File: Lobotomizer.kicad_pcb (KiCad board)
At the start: 2 copper layers, 134 x 101.6 mm, 170 parts, among them J1 IN, J2 OUT, J3 Barrel_Jack, Q1 NTE467, Q2 2N5089, Q201 MPSA05, Q202 MPSA05, Q3 2N5087, Q4 2N5089, Q5 NTE467, Q6 BS170, SW1 SW_SPDT_MSM, SW101 SW_Push_DPDT, SW102 SW_SPDT, SW2 SW_SPDT, SW201 SW_SPDT, SW202 SW_SPDT, SW3 SW_SPDT, U1 LM741, U101 TLC27M4AIN, U102 BTDR-2H-L, U103 L7805, U201 LM386, U202 TL072

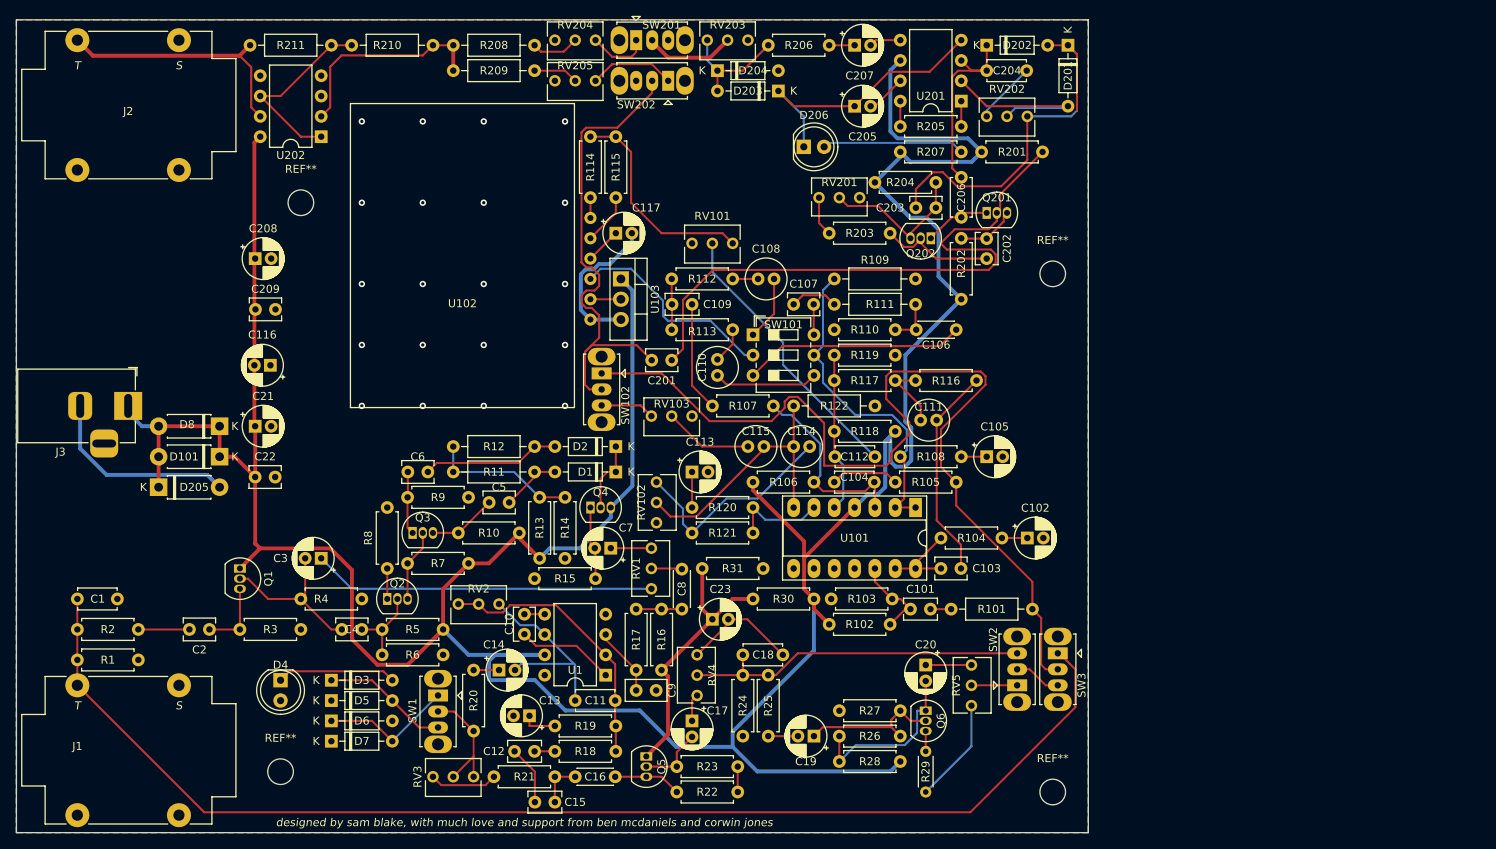
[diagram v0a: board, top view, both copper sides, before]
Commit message: lobotomizer v2 update
so much changed i cant note it all here
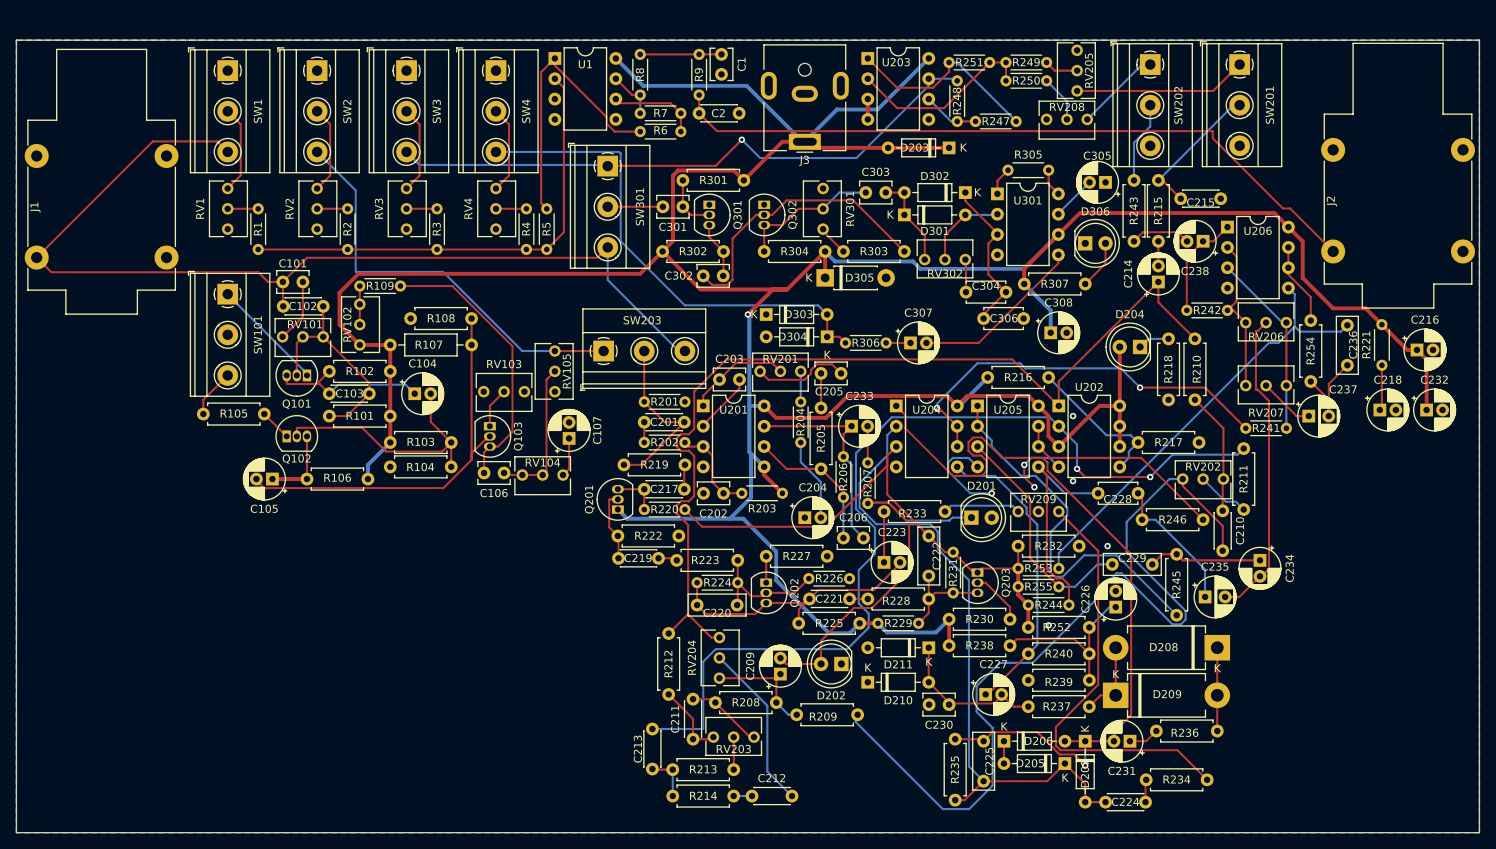
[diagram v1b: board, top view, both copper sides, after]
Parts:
- removed C10: 30p, Capacitor_THT:C_Rect_L4.0mm_W2.5mm_P2.50mm
- removed C108, C110, C115: 220n, Capacitor_THT:C_Radial_D5.0mm_H11.0mm_P2.00mm
- removed C109: 33n, Capacitor_THT:C_Rect_L4.0mm_W2.5mm_P2.50mm
- removed C11, C18: 100p, Capacitor_THT:C_Disc_D4.7mm_W2.5mm_P5.00mm
- removed C111, C114: 470p, Capacitor_THT:C_Radial_D5.0mm_H11.0mm_P2.00mm
- removed C112: 10n, Capacitor_THT:C_Disc_D4.7mm_W2.5mm_P5.00mm
- removed C113, C17, C19, C3, C7: 1u, Capacitor_THT:CP_Radial_D5.0mm_P2.00mm
- removed C116, C117, C207, C208, C21: 100u, Capacitor_THT:CP_Radial_D5.0mm_P2.00mm
- removed C12: 2.2p, Capacitor_THT:C_Rect_L4.0mm_W2.5mm_P2.50mm
- removed C13, C14: 4.7u, Capacitor_THT:CP_Radial_D5.0mm_P2.00mm
- removed C15: 3.3n, Capacitor_THT:C_Rect_L4.0mm_W2.5mm_P2.50mm
- removed C16, C8: 22n, Capacitor_THT:C_Disc_D4.3mm_W1.9mm_P5.00mm
- removed C20, C23: 10u, Capacitor_THT:CP_Radial_D5.0mm_P2.00mm
- removed C22, C4, C5, C6: 100n, Capacitor_THT:C_Disc_D3.8mm_W2.6mm_P2.50mm
- removed C9: 1n, Capacitor_THT:C_Disc_D5.0mm_W2.5mm_P2.50mm
- removed D1, D2, D3, D5, D6, D7: 4148, Diode_THT:D_DO-35_SOD27_P7.62mm_Horizontal
- removed D101: 4001, Diode_THT:D_DO-41_SOD81_P7.62mm_Horizontal
- removed D4: LED, LED_THT:LED_D5.0mm
- removed D8: 5817, Diode_THT:D_DO-41_SOD81_P7.62mm_Horizontal
- removed G***: LOGO, BSilk:Lobotomizer
- removed Q1, Q5: NTE467, Package_TO_SOT_THT:TO-92_Inline
- removed Q2, Q4: 2N5089, Package_TO_SOT_THT:TO-92_Inline
- removed Q3: 2N5087, Package_TO_SOT_THT:TO-92_Inline
- removed Q6: BS170, Package_TO_SOT_THT:TO-92_Inline
- removed R10, R120, R15, R23, R28, R30, R31: 10K, Resistor_THT:R_Axial_DIN0207_L6.3mm_D2.5mm_P7.62mm_Horizontal
- removed R11, R111, R12, R122: 100K, Resistor_THT:R_Axial_DIN0207_L6.3mm_D2.5mm_P10.16mm_Horizontal
- removed R110, R17, R20, R25: 1K, Resistor_THT:R_Axial_DIN0207_L6.3mm_D2.5mm_P7.62mm_Horizontal
- removed R112, R113: 39K, Resistor_THT:R_Axial_DIN0207_L6.3mm_D2.5mm_P7.62mm_Horizontal
- removed R114, R115: 5K, Resistor_THT:R_Axial_DIN0207_L6.3mm_D2.5mm_P7.62mm_Horizontal
- removed R116, R118, R119, R16, R22, R24: 1M, Resistor_THT:R_Axial_DIN0207_L6.3mm_D2.5mm_P7.62mm_Horizontal
- removed R117: 6.8K, Resistor_THT:R_Axial_DIN0207_L6.3mm_D2.5mm_P7.62mm_Horizontal
- removed R121: 68K, Resistor_THT:R_Axial_DIN0207_L6.3mm_D2.5mm_P7.62mm_Horizontal
- removed R13, R14: 47K, Resistor_THT:R_Axial_DIN0207_L6.3mm_D2.5mm_P7.62mm_Horizontal
- removed R18: 47, Resistor_THT:R_Axial_DIN0207_L6.3mm_D2.5mm_P7.62mm_Horizontal
- removed R19: 560, Resistor_THT:R_Axial_DIN0207_L6.3mm_D2.5mm_P7.62mm_Horizontal
- removed R21: 1.5K, Resistor_THT:R_Axial_DIN0207_L6.3mm_D2.5mm_P7.62mm_Horizontal
- removed R26, R27: 470K, Resistor_THT:R_Axial_DIN0207_L6.3mm_D2.5mm_P7.62mm_Horizontal
- removed R29: 470, Resistor_THT:R_Axial_DIN0204_L3.6mm_D1.6mm_P5.08mm_Horizontal
- removed REF** (x4): MountingHole_3.2mm_M3, MountingHole:MountingHole_3.2mm_M3
- removed RV5: 100K, Potentiometer_THT:Potentiometer_Bourns_3266Y_Vertical
- removed SW102: SW_SPDT, Button_Switch_THT:SW_Slide_1P2T_CK_OS102011MS2Q
- removed U101: TLC27M4AIN, Package_DIP:DIP-14_W7.62mm_Socket_LongPads
- removed U102: BTDR-2H-L, Lobotomizer:BTDR-2H-L
- removed U103: L7805, Package_TO_SOT_THT:TO-220-3_Vertical
- added C210: 47n, Capacitor_THT:C_Disc_D4.3mm_W1.9mm_P5.00mm, F.Cu at (227.0, 112.2)
- added C211: 10n, Capacitor_THT:C_Disc_D4.3mm_W1.9mm_P5.00mm, F.Cu at (160.8, 140.7)
- added C212: 2.2n, Capacitor_THT:C_Disc_D4.3mm_W1.9mm_P5.00mm, F.Cu at (168.1, 147.8)
- added C213: 10n, Capacitor_THT:C_Disc_D4.3mm_W1.9mm_P5.00mm, F.Cu at (155.7, 139.4)
- added C214: 2.2u, Capacitor_THT:CP_Radial_D5.0mm_P2.00mm, F.Cu at (218.9, 83.6)
- added C215: 22n, Capacitor_THT:C_Disc_D4.3mm_W1.9mm_P5.00mm, F.Cu at (221.7, 73.2)
- added C216: 100u, Capacitor_THT:CP_Radial_D5.0mm_P2.00mm, F.Cu at (251.3, 92.1)
- added C217: 47n, Capacitor_THT:C_Disc_D4.3mm_W1.9mm_P5.00mm, F.Cu at (154.7, 109.5)
- added C218: 47u, Capacitor_THT:CP_Radial_D5.0mm_P2.00mm, F.Cu at (246.6, 99.6)
- added C219: 47n, Capacitor_THT:C_Disc_D4.3mm_W1.9mm_P5.00mm, F.Cu at (156.5, 118.1)
- added C220: 10p, Capacitor_THT:C_Disc_D7.0mm_W2.5mm_P5.00mm, F.Cu at (161.3, 124.0)
- added C221: 47n, Capacitor_THT:C_Disc_D4.3mm_W1.9mm_P5.00mm, F.Cu at (180.3, 123.2)
- added C222: 10p, Capacitor_THT:C_Disc_D7.0mm_W2.5mm_P5.00mm, F.Cu at (190.2, 115.3)
- added C223: 10u, Capacitor_THT:CP_Radial_D5.0mm_P2.00mm, F.Cu at (184.7, 118.6)
- added C224: 47n, Capacitor_THT:C_Disc_D4.3mm_W1.9mm_P5.00mm, F.Cu at (212.3, 148.6)
- added C225: 10p, Capacitor_THT:C_Disc_D7.0mm_W2.5mm_P5.00mm, F.Cu at (197.1, 141.0)
- added C226: 47u, Capacitor_THT:CP_Radial_D5.0mm_P2.00mm, F.Cu at (213.6, 124.2)
- added C227: 1u, Capacitor_THT:CP_Radial_D5.0mm_P2.00mm, F.Cu at (197.4, 135.1)
- added C228: 6.8n, Capacitor_THT:C_Disc_D4.7mm_W2.5mm_P5.00mm, F.Cu at (216.4, 110.0)
- added C229: 4.7n, Capacitor_THT:C_Disc_D7.0mm_W2.5mm_P5.00mm, F.Cu at (218.2, 118.9)
- added C230: 1n, Capacitor_THT:C_Disc_D3.8mm_W2.6mm_P2.50mm, F.Cu at (192.8, 136.4)
- added C231: 1u, Capacitor_THT:CP_Radial_D5.0mm_P2.00mm, F.Cu at (215.4, 141.0)
- added C232: 100u, Capacitor_THT:CP_Radial_D5.0mm_P2.00mm, F.Cu at (252.5, 99.6)
- added C233: 2.2u, Capacitor_THT:CP_Radial_D5.0mm_P2.00mm, F.Cu at (180.6, 101.6)
- added C234: 0.1u, Capacitor_THT:CP_Radial_D5.0mm_P2.00mm, F.Cu at (231.6, 118.4)
- added C235: 0.15u, Capacitor_THT:CP_Radial_D5.0mm_P2.50mm, F.Cu at (224.8, 122.9)
- added C236: 68n, Capacitor_THT:C_Disc_D7.0mm_W2.5mm_P5.00mm, F.Cu at (242.6, 94.0)
- added C237: 1.5u, Capacitor_THT:CP_Radial_D5.0mm_P2.50mm, F.Cu at (237.7, 100.3)
- added C238: 10u, Capacitor_THT:CP_Radial_D5.0mm_P2.00mm, F.Cu at (224.5, 78.5)
- added C301: 100n, Capacitor_THT:C_Disc_D3.8mm_W2.6mm_P2.50mm, F.Cu at (159.5, 74.2)
- added C302: 100n, Capacitor_THT:C_Disc_D3.8mm_W2.6mm_P2.50mm, F.Cu at (162.1, 82.8)
- added C303: 100n, Capacitor_THT:C_Disc_D3.8mm_W2.6mm_P2.50mm, F.Cu at (182.4, 72.4)
- added C304: 6.8n, Capacitor_THT:C_Disc_D4.7mm_W2.5mm_P5.00mm, F.Cu at (199.9, 84.8)
- added C305: 4.7u, Capacitor_THT:CP_Radial_D5.0mm_P2.00mm, F.Cu at (212.3, 71.1)
- added C306: 220p, Capacitor_THT:C_Disc_D4.7mm_W2.5mm_P5.00mm, F.Cu at (197.1, 88.1)
- added C307: 100u, Capacitor_THT:CP_Radial_D5.0mm_P2.00mm, F.Cu at (188.0, 91.2)
- added C308: 100u, Capacitor_THT:CP_Radial_D5.0mm_P2.00mm, F.Cu at (205.5, 89.9)
- added D207: 4148, Diode_THT:D_DO-35_SOD27_P7.62mm_Horizontal, F.Cu at (209.8, 141.0)
- added D208: SB2060, Diode_THT:D_DO-201AD_P12.70mm_Horizontal, F.Cu at (226.3, 129.3)
- added D209: SB2060, Diode_THT:D_DO-201AD_P12.70mm_Horizontal, F.Cu at (213.6, 135.2)
- added D210: 4148, Diode_THT:D_DO-35_SOD27_P7.62mm_Horizontal, F.Cu at (182.6, 133.6)
- added D211: 4148, Diode_THT:D_DO-35_SOD27_P7.62mm_Horizontal, F.Cu at (190.2, 129.3)
- added D301: 5227, Diode_THT:D_DO-35_SOD27_P7.62mm_Horizontal, F.Cu at (187.2, 75.2)
- added D302: 5227, Diode_THT:D_DO-35_SOD27_P7.62mm_Horizontal, F.Cu at (194.8, 72.4)
- added D303: 5227, Diode_THT:D_DO-35_SOD27_P7.62mm_Horizontal, F.Cu at (169.9, 87.6)
- added D304: 5227, Diode_THT:D_DO-35_SOD27_P7.62mm_Horizontal, F.Cu at (177.5, 90.4)
- added D305: 4001, Diode_THT:D_DO-41_SOD81_P7.62mm_Horizontal, F.Cu at (177.3, 83.1)
- added D306: LED, LED_THT:LED_D5.0mm, F.Cu at (209.8, 78.7)
- added Q101: 5089, Package_TO_SOT_THT:TO-92_Inline, F.Cu at (112.5, 95.2)
- added Q102: 5089, Package_TO_SOT_THT:TO-92_Inline, F.Cu at (110.0, 102.9)
- added Q103: 5308, Package_TO_SOT_THT:TO-92_Inline, F.Cu at (135.4, 101.6)
- added Q203: KSA992, Package_TO_SOT_THT:TO-92_Inline, F.Cu at (196.3, 119.9)
- added Q301: MPSA05, Package_TO_SOT_THT:TO-92_Inline, F.Cu at (162.8, 73.9)
- added Q302: MPSA05, Package_TO_SOT_THT:TO-92_Inline, F.Cu at (169.7, 73.9)
- added R212: 2.2K, Resistor_THT:R_Axial_DIN0207_L6.3mm_D2.5mm_P7.62mm_Horizontal, F.Cu at (157.7, 127.5)
- added R213: 15K, Resistor_THT:R_Axial_DIN0207_L6.3mm_D2.5mm_P7.62mm_Horizontal, F.Cu at (158.2, 144.5)
- added R214: 10K, Resistor_THT:R_Axial_DIN0207_L6.3mm_D2.5mm_P7.62mm_Horizontal, F.Cu at (158.2, 147.8)
- added R215: 6.8K, Resistor_THT:R_Axial_DIN0207_L6.3mm_D2.5mm_P7.62mm_Horizontal, F.Cu at (218.9, 70.9)
- added R216: 22K, Resistor_THT:R_Axial_DIN0207_L6.3mm_D2.5mm_P7.62mm_Horizontal, F.Cu at (197.6, 95.5)
- added R217: 22K, Resistor_THT:R_Axial_DIN0207_L6.3mm_D2.5mm_P7.62mm_Horizontal, F.Cu at (216.4, 103.6)
- added R218: 4.7K, Resistor_THT:R_Axial_DIN0207_L6.3mm_D2.5mm_P7.62mm_Horizontal, F.Cu at (220.2, 98.3)
- added R219: 10K, Resistor_THT:R_Axial_DIN0207_L6.3mm_D2.5mm_P7.62mm_Horizontal, F.Cu at (159.8, 106.4)
- added R220: 1M, Resistor_THT:R_Axial_DIN0204_L3.6mm_D1.6mm_P5.08mm_Horizontal, F.Cu at (159.8, 112.0)
- added R221: 1K, Resistor_THT:R_Axial_DIN0204_L3.6mm_D1.6mm_P5.08mm_Horizontal, F.Cu at (246.9, 94.0)
- added R222: 10K, Resistor_THT:R_Axial_DIN0207_L6.3mm_D2.5mm_P7.62mm_Horizontal, F.Cu at (151.4, 115.3)
- added R223: 22K, Resistor_THT:R_Axial_DIN0207_L6.3mm_D2.5mm_P7.62mm_Horizontal, F.Cu at (166.4, 118.4)
- added R224: 470K, Resistor_THT:R_Axial_DIN0204_L3.6mm_D1.6mm_P5.08mm_Horizontal, F.Cu at (161.3, 121.2)
- added R225: 10K, Resistor_THT:R_Axial_DIN0207_L6.3mm_D2.5mm_P7.62mm_Horizontal, F.Cu at (181.6, 126.2)
- added R226: 100K, Resistor_THT:R_Axial_DIN0204_L3.6mm_D1.6mm_P5.08mm_Horizontal, F.Cu at (175.3, 120.7)
- added R227: 22, Resistor_THT:R_Axial_DIN0207_L6.3mm_D2.5mm_P7.62mm_Horizontal, F.Cu at (169.9, 117.9)
- added R228: 22K, Resistor_THT:R_Axial_DIN0207_L6.3mm_D2.5mm_P7.62mm_Horizontal, F.Cu at (190.2, 123.2)
- added R229: 100K, Resistor_THT:R_Axial_DIN0204_L3.6mm_D1.6mm_P5.08mm_Horizontal, F.Cu at (183.9, 126.2)
- added R230: 120, Resistor_THT:R_Axial_DIN0207_L6.3mm_D2.5mm_P7.62mm_Horizontal, F.Cu at (192.8, 125.7)
- added R231: 470K, Resistor_THT:R_Axial_DIN0204_L3.6mm_D1.6mm_P5.08mm_Horizontal, F.Cu at (193.3, 117.3)
- added R232: 10K, Resistor_THT:R_Axial_DIN0207_L6.3mm_D2.5mm_P7.62mm_Horizontal, F.Cu at (201.4, 116.6)
- added R233: 150, Resistor_THT:R_Axial_DIN0207_L6.3mm_D2.5mm_P7.62mm_Horizontal, F.Cu at (192.3, 112.3)
- added R234: 47K, Resistor_THT:R_Axial_DIN0207_L6.3mm_D2.5mm_P7.62mm_Horizontal, F.Cu at (217.4, 145.8)
- added R235: 220K, Resistor_THT:R_Axial_DIN0207_L6.3mm_D2.5mm_P7.62mm_Horizontal, F.Cu at (193.5, 140.7)
- added R236: 10K, Resistor_THT:R_Axial_DIN0207_L6.3mm_D2.5mm_P7.62mm_Horizontal, F.Cu at (226.3, 139.7)
- added R237: 10K, Resistor_THT:R_Axial_DIN0207_L6.3mm_D2.5mm_P7.62mm_Horizontal, F.Cu at (202.7, 136.7)
- added R238: 10K, Resistor_THT:R_Axial_DIN0207_L6.3mm_D2.5mm_P7.62mm_Horizontal, F.Cu at (192.8, 129.0)
- added R239: 10K, Resistor_THT:R_Axial_DIN0207_L6.3mm_D2.5mm_P7.62mm_Horizontal, F.Cu at (210.3, 133.3)
- added R240: 68K, Resistor_THT:R_Axial_DIN0207_L6.3mm_D2.5mm_P7.62mm_Horizontal, F.Cu at (210.3, 130.0)
- added R241: 3.3K, Resistor_THT:R_Axial_DIN0204_L3.6mm_D1.6mm_P5.08mm_Horizontal, F.Cu at (234.9, 101.9)
- added R242: 3.3K, Resistor_THT:R_Axial_DIN0204_L3.6mm_D1.6mm_P5.08mm_Horizontal, F.Cu at (222.5, 87.1)
- added R243: 10K, Resistor_THT:R_Axial_DIN0207_L6.3mm_D2.5mm_P7.62mm_Horizontal, F.Cu at (215.9, 70.9)
- added R244: 100K, Resistor_THT:R_Axial_DIN0204_L3.6mm_D1.6mm_P5.08mm_Horizontal, F.Cu at (207.8, 124.0)
- added R245: 330, Resistor_THT:R_Axial_DIN0207_L6.3mm_D2.5mm_P7.62mm_Horizontal, F.Cu at (221.2, 117.6)
- added R246: 330, Resistor_THT:R_Axial_DIN0207_L6.3mm_D2.5mm_P7.62mm_Horizontal, F.Cu at (216.9, 113.3)
- added R247: 100K, Resistor_THT:R_Axial_DIN0204_L3.6mm_D1.6mm_P5.08mm_Horizontal, F.Cu at (196.1, 63.5)
- added R248: 100K, Resistor_THT:R_Axial_DIN0204_L3.6mm_D1.6mm_P5.08mm_Horizontal, F.Cu at (193.8, 58.4)
- added R249: 100K, Resistor_THT:R_Axial_DIN0204_L3.6mm_D1.6mm_P5.08mm_Horizontal, F.Cu at (199.9, 56.1)
- added R250: 100K, Resistor_THT:R_Axial_DIN0204_L3.6mm_D1.6mm_P5.08mm_Horizontal, F.Cu at (199.9, 58.4)
- added R251: 100K, Resistor_THT:R_Axial_DIN0204_L3.6mm_D1.6mm_P5.08mm_Horizontal, F.Cu at (192.8, 56.1)
- added R252: 68K, Resistor_THT:R_Axial_DIN0207_L6.3mm_D2.5mm_P7.62mm_Horizontal, F.Cu at (210.3, 126.7)
- added R253: 100K, Resistor_THT:R_Axial_DIN0204_L3.6mm_D1.6mm_P5.08mm_Horizontal, F.Cu at (206.5, 119.4)
- added R254: 330, Resistor_THT:R_Axial_DIN0207_L6.3mm_D2.5mm_P7.62mm_Horizontal, F.Cu at (238.0, 96.0)
- added R255: 100K, Resistor_THT:R_Axial_DIN0204_L3.6mm_D1.6mm_P5.08mm_Horizontal, F.Cu at (206.5, 121.7)
- added R301: 910K, Resistor_THT:R_Axial_DIN0207_L6.3mm_D2.5mm_P7.62mm_Horizontal, F.Cu at (167.1, 70.9)
- added R302: 180K, Resistor_THT:R_Axial_DIN0207_L6.3mm_D2.5mm_P7.62mm_Horizontal, F.Cu at (157.0, 79.8)
- added R303: 4.7K, Resistor_THT:R_Axial_DIN0207_L6.3mm_D2.5mm_P7.62mm_Horizontal, F.Cu at (187.2, 79.8)
- added R304: 180K, Resistor_THT:R_Axial_DIN0207_L6.3mm_D2.5mm_P7.62mm_Horizontal, F.Cu at (177.3, 79.8)
- added R305: 1K, Resistor_THT:R_Axial_DIN0204_L3.6mm_D1.6mm_P5.08mm_Horizontal, F.Cu at (200.2, 69.6)
- added R306: 220, Resistor_THT:R_Axial_DIN0204_L3.6mm_D1.6mm_P5.08mm_Horizontal, F.Cu at (179.8, 91.2)
- added R307: 10K, Resistor_THT:R_Axial_DIN0207_L6.3mm_D2.5mm_P7.62mm_Horizontal, F.Cu at (209.8, 83.8)
- added RV104: 10K, Potentiometer_THT:Potentiometer_Bourns_3266Y_Vertical, F.Cu at (144.5, 107.7)
- added RV105: 100K, Potentiometer_THT:Potentiometer_Bourns_3266Y_Vertical, F.Cu at (143.5, 97.3)
- added RV206: 10K, Potentiometer_THT:Potentiometer_Bourns_3266Y_Vertical, F.Cu at (229.9, 88.6)
- added RV207: 10K, Potentiometer_THT:Potentiometer_Bourns_3266Y_Vertical, F.Cu at (229.9, 96.5)
- added RV208: 10K, Potentiometer_THT:Potentiometer_Bourns_3266Y_Vertical, F.Cu at (210.1, 63.2)
- added RV209: 250K, Potentiometer_THT:Potentiometer_Bourns_3266Y_Vertical, F.Cu at (206.5, 112.3)
- added RV301: 1M, Potentiometer_THT:Potentiometer_Bourns_3266Y_Vertical, F.Cu at (177.0, 77.0)
- added RV302: 1M, Potentiometer_THT:Potentiometer_Bourns_3266Y_Vertical, F.Cu at (189.7, 80.8)
- added SW203: SW_SPDT, TerminalBlock_Phoenix:TerminalBlock_Phoenix_MKDS-1,5-3-5.08_1x03_P5.08mm_Horizontal, F.Cu at (149.6, 92.2)
- added SW301: SW_SPDT, TerminalBlock_Phoenix:TerminalBlock_Phoenix_MKDS-1,5-3-5.08_1x03_P5.08mm_Horizontal, F.Cu at (150.1, 69.1)
- added SW4: SW_SPDT, TerminalBlock_Phoenix:TerminalBlock_Phoenix_MKDS-1,5-3-5.08_1x03_P5.08mm_Horizontal, F.Cu at (136.1, 57.1)
- added U203: TL082, Package_DIP:DIP-8_W7.62mm, F.Cu at (182.6, 55.6)
- added U204: LM833, Package_DIP:DIP-8_W7.62mm, F.Cu at (186.2, 99.1)
- added U205: LM833, Package_DIP:DIP-8_W7.62mm, F.Cu at (196.3, 99.1)
- added U206: LM833, Package_DIP:DIP-8_W7.62mm, F.Cu at (227.6, 76.7)
- added U301: LM386, Package_DIP:DIP-8_W7.62mm, F.Cu at (198.8, 72.6)
- C1: value 100p -> 1n; footprint Capacitor_THT:C_Disc_D4.7mm_W2.5mm_P5.00mm -> Capacitor_THT:C_Disc_D3.8mm_W2.6mm_P2.50mm
- C101: value 33n -> 100n; footprint Capacitor_THT:C_Rect_L4.0mm_W2.5mm_P2.50mm -> Capacitor_THT:C_Disc_D3.8mm_W2.6mm_P2.50mm
- C102: value 1u -> 10n; footprint Capacitor_THT:CP_Radial_D5.0mm_P2.00mm -> Capacitor_THT:C_Disc_D4.3mm_W1.9mm_P5.00mm
- C103: value 100n -> 470p; footprint Capacitor_THT:C_Disc_D3.8mm_W2.6mm_P2.50mm -> Capacitor_THT:C_Disc_D4.3mm_W1.9mm_P5.00mm
- C104: value 10n -> 4.7u; footprint Capacitor_THT:C_Disc_D4.7mm_W2.5mm_P5.00mm -> Capacitor_THT:CP_Radial_D5.0mm_P2.00mm
- C105: value 1u -> 4.7u
- C106: value 4.7n -> 100n; footprint Capacitor_THT:C_Disc_D4.3mm_W1.9mm_P5.00mm -> Capacitor_THT:C_Disc_D3.8mm_W2.6mm_P2.50mm
- C107: value 100n -> 330n; footprint Capacitor_THT:C_Disc_D3.8mm_W2.6mm_P2.50mm -> Capacitor_THT:CP_Radial_D5.0mm_P2.00mm
- C2: value 100n -> 680p; footprint Capacitor_THT:C_Disc_D3.8mm_W2.6mm_P2.50mm -> Capacitor_THT:C_Disc_D4.3mm_W1.9mm_P5.00mm
- C201: value 100n -> 22n; footprint Capacitor_THT:C_Disc_D3.8mm_W2.6mm_P2.50mm -> Capacitor_THT:C_Disc_D4.3mm_W1.9mm_P5.00mm
- C202: value 100n -> 1n
- C203: value 100n -> 100p
- C204: value 6.8n -> 220n; footprint Capacitor_THT:C_Disc_D4.7mm_W2.5mm_P5.00mm -> Capacitor_THT:CP_Radial_D5.0mm_P2.00mm
- C205: value 4.7u -> 100n; footprint Capacitor_THT:CP_Radial_D5.0mm_P2.00mm -> Capacitor_THT:C_Disc_D3.8mm_W2.6mm_P2.50mm
- C206: value 220p -> 100p; footprint Capacitor_THT:C_Disc_D4.7mm_W2.5mm_P5.00mm -> Capacitor_THT:C_Disc_D3.8mm_W2.6mm_P2.50mm
- C209: value 100n -> 2.2u; footprint Capacitor_THT:C_Disc_D3.8mm_W2.6mm_P2.50mm -> Capacitor_THT:CP_Radial_D5.0mm_P2.00mm
- D201, D202, D204: value 5227 -> LED; footprint Diode_THT:D_DO-35_SOD27_P7.62mm_Horizontal -> LED_THT:LED_D5.0mm
- D203: value 5227 -> 4148
- D205: value 4001 -> 4148; footprint Diode_THT:D_DO-41_SOD81_P7.62mm_Horizontal -> Diode_THT:D_DO-35_SOD27_P7.62mm_Horizontal
- D206: value LED -> 4148; footprint LED_THT:LED_D5.0mm -> Diode_THT:D_DO-35_SOD27_P7.62mm_Horizontal
- J1, J2: footprint Connector_Audio:Jack_6.35mm_Neutrik_NMJ4HCD2_Horizontal -> Connector_Audio:Jack_6.35mm_Neutrik_NMJ4HFD2_Horizontal
- J3: value Barrel_Jack -> POWER; footprint Connector_BarrelJack:BarrelJack_Horizontal -> Connector_BarrelJack:BarrelJack_CUI_PJ-063AH_Horizontal
- Q201: value MPSA05 -> NTE457
- Q202: value MPSA05 -> 2N3904
- R1, R3: value 1M -> 100K; footprint Resistor_THT:R_Axial_DIN0207_L6.3mm_D2.5mm_P7.62mm_Horizontal -> Resistor_THT:R_Axial_DIN0204_L3.6mm_D1.6mm_P5.08mm_Horizontal
- R101: value 100K -> 910K; footprint Resistor_THT:R_Axial_DIN0207_L6.3mm_D2.5mm_P10.16mm_Horizontal -> Resistor_THT:R_Axial_DIN0207_L6.3mm_D2.5mm_P7.62mm_Horizontal
- R102, R106: value 1M -> 180K
- R103: value 1M -> 910K
- R104: value 10K -> 910
- R107: value 1M -> 4.7M; footprint Resistor_THT:R_Axial_DIN0207_L6.3mm_D2.5mm_P7.62mm_Horizontal -> Resistor_THT:R_Axial_DIN0207_L6.3mm_D2.5mm_P10.16mm_Horizontal
- R108: value 10K -> 910K
- R109: value 100K -> 750; footprint Resistor_THT:R_Axial_DIN0207_L6.3mm_D2.5mm_P10.16mm_Horizontal -> Resistor_THT:R_Axial_DIN0204_L3.6mm_D1.6mm_P5.08mm_Horizontal
- R2, R4: value 1K -> 100K; footprint Resistor_THT:R_Axial_DIN0207_L6.3mm_D2.5mm_P7.62mm_Horizontal -> Resistor_THT:R_Axial_DIN0204_L3.6mm_D1.6mm_P5.08mm_Horizontal
- R201: value 910K -> 1M; footprint Resistor_THT:R_Axial_DIN0207_L6.3mm_D2.5mm_P7.62mm_Horizontal -> Resistor_THT:R_Axial_DIN0204_L3.6mm_D1.6mm_P5.08mm_Horizontal
- R202, R204: value 180K -> 1K; footprint Resistor_THT:R_Axial_DIN0207_L6.3mm_D2.5mm_P7.62mm_Horizontal -> Resistor_THT:R_Axial_DIN0204_L3.6mm_D1.6mm_P5.08mm_Horizontal
- R203: value 4.7K -> 1M; footprint Resistor_THT:R_Axial_DIN0207_L6.3mm_D2.5mm_P7.62mm_Horizontal -> Resistor_THT:R_Axial_DIN0204_L3.6mm_D1.6mm_P5.08mm_Horizontal
- R205: value 1K -> 10K
- R206: value 220 -> 1M; footprint Resistor_THT:R_Axial_DIN0207_L6.3mm_D2.5mm_P7.62mm_Horizontal -> Resistor_THT:R_Axial_DIN0204_L3.6mm_D1.6mm_P5.08mm_Horizontal
- R207: value 10K -> 470; footprint Resistor_THT:R_Axial_DIN0207_L6.3mm_D2.5mm_P7.62mm_Horizontal -> Resistor_THT:R_Axial_DIN0204_L3.6mm_D1.6mm_P5.08mm_Horizontal
- R208: value 100K -> 2.2K; footprint Resistor_THT:R_Axial_DIN0207_L6.3mm_D2.5mm_P10.16mm_Horizontal -> Resistor_THT:R_Axial_DIN0207_L6.3mm_D2.5mm_P7.62mm_Horizontal
- R209, R210: value 100K -> 6.8K; footprint Resistor_THT:R_Axial_DIN0207_L6.3mm_D2.5mm_P10.16mm_Horizontal -> Resistor_THT:R_Axial_DIN0207_L6.3mm_D2.5mm_P7.62mm_Horizontal
- R211: value 100K -> 68K; footprint Resistor_THT:R_Axial_DIN0207_L6.3mm_D2.5mm_P10.16mm_Horizontal -> Resistor_THT:R_Axial_DIN0207_L6.3mm_D2.5mm_P7.62mm_Horizontal
- R5: value 470K -> 100K; footprint Resistor_THT:R_Axial_DIN0207_L6.3mm_D2.5mm_P7.62mm_Horizontal -> Resistor_THT:R_Axial_DIN0204_L3.6mm_D1.6mm_P5.08mm_Horizontal
- R6: value 47K -> 100K; footprint Resistor_THT:R_Axial_DIN0207_L6.3mm_D2.5mm_P7.62mm_Horizontal -> Resistor_THT:R_Axial_DIN0204_L3.6mm_D1.6mm_P5.08mm_Horizontal
- R7: value 22K -> 100K; footprint Resistor_THT:R_Axial_DIN0207_L6.3mm_D2.5mm_P7.62mm_Horizontal -> Resistor_THT:R_Axial_DIN0204_L3.6mm_D1.6mm_P5.08mm_Horizontal
- R8: value 2.2K -> 100K; footprint Resistor_THT:R_Axial_DIN0207_L6.3mm_D2.5mm_P7.62mm_Horizontal -> Resistor_THT:R_Axial_DIN0204_L3.6mm_D1.6mm_P5.08mm_Horizontal
- R9: value 10K -> 100K; footprint Resistor_THT:R_Axial_DIN0207_L6.3mm_D2.5mm_P7.62mm_Horizontal -> Resistor_THT:R_Axial_DIN0204_L3.6mm_D1.6mm_P5.08mm_Horizontal
- RV1: value 50K -> 100K
- RV101: value 10K -> 100K
- RV102: value 1M -> 50K
- RV103: value 100K -> 10K
- RV201: value 1M -> 100K
- RV202: value 1M -> 25K
- RV203: value 100K -> 25K
- SW1: value SW_SPDT_MSM -> SW_SPDT; footprint Button_Switch_THT:SW_Slide_1P2T_CK_OS102011MS2Q -> TerminalBlock_Phoenix:TerminalBlock_Phoenix_MKDS-1,5-3-5.08_1x03_P5.08mm_Horizontal
- SW101: value SW_Push_DPDT -> SW_SPDT_MSM; footprint Button_Switch_THT:SW_DIP_SPSTx03_Slide_6.7x9.18mm_W7.62mm_P2.54mm_LowProfile -> TerminalBlock_Phoenix:TerminalBlock_Phoenix_MKDS-1,5-3-5.08_1x03_P5.08mm_Horizontal
- SW2, SW201, SW202, SW3: footprint Button_Switch_THT:SW_Slide_1P2T_CK_OS102011MS2Q -> TerminalBlock_Phoenix:TerminalBlock_Phoenix_MKDS-1,5-3-5.08_1x03_P5.08mm_Horizontal
- U1: value LM741 -> TL082
- U201: value LM386 -> LM833
- U202: value TL072 -> TL082
- moved J2 159.2 mm to (240.8, 79.8), turned to 90 degrees
- moved R211 134.0 mm to (229.6, 104.4), turned to 270 degrees
- moved D205 118.4 mm to (207.3, 143.8), turned to 180 degrees
- moved SW2 116.4 mm to (113.8, 57.1), turned to 270 degrees
- moved R210 111.6 mm to (223.5, 90.7), turned to 270 degrees
- moved SW3 109.2 mm to (125.0, 57.1)
- moved C1 105.4 mm to (164.3, 55.1), turned to 270 degrees
- moved U202 98.2 mm to (206.5, 99.1), turned to 0 degrees
- moved R209 95.1 mm to (181.4, 137.7), turned to 180 degrees
- moved R105 94.5 mm to (99.6, 100.1), turned to 0 degrees
- moved C102 92.7 mm to (114.6, 86.6), turned to 180 degrees
- moved J3 90.8 mm to (174.8, 66.0), turned to 180 degrees
- moved C105 89.3 mm to (108.2, 108.2), turned to 180 degrees
- moved C2 88.9 mm to (161.5, 62.5), turned to 0 degrees
- moved R208 88.5 mm to (163.6, 136.1)
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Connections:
- C1 pad 1: BYPASS_FUZZ -> Net-(C1-Pad1)
- C101 pad 2: Net-(C101-Pad2) -> SIGNAL_IN
- C102 pad 2: GND -> SIGNAL_IN
- C103 pad 2: Net-(C103-Pad2) -> Net-(C102-Pad1)
- C104 pad 1: Net-(C104-Pad1) -> Net-(C103-Pad1)
- C105 pad 2: GND -> Net-(C105-Pad2)
- C107 pad 2: Net-(C107-Pad2) -> GND
- C2 pad 2: Net-(C2-Pad2) -> GND
- C201 pad 2: REVERB_OUT -> Net-(C201-Pad2)
- C202 pad 2: Net-(C202-Pad2) -> GND
- C204 pad 1: Net-(C204-Pad1) -> GND
- C205 pad 1: GND -> Net-(C205-Pad1)
- C206 pad 1: Net-(C204-Pad1) -> Net-(C206-Pad1)
- C206 pad 2: GND -> Net-(C206-Pad2)
- C209 pad 1: GND -> Net-(C209-Pad1)
- C209 pad 2: VCLEAN -> Net-(C209-Pad2)
- D201 pad 1: Net-(C203-Pad2) -> Net-(C209-Pad2)
- D201 pad 2: Net-(D201-Pad2) -> GND
- D202 pad 1: Net-(C204-Pad1) -> GND
- D202 pad 2: Net-(C203-Pad2) -> Net-(C209-Pad2)
- D203 pad 1: GND -> VCLEAN
- D203 pad 2: Net-(D203-Pad2) -> VCLEAN
- D204 pad 1: Net-(D203-Pad2) -> Net-(D204-Pad1)
- D204 pad 2: GND -> VCLEAN
- D205 pad 1: VCLEAN -> Net-(C224-Pad1)
- D205 pad 2: GND -> Net-(D205-Pad2)
- D206 pad 1: GND -> Net-(D205-Pad2)
- D206 pad 2: Net-(D206-Pad2) -> Net-(C225-Pad1)
- J1 pad T: BYPASS_FUZZ -> SIGNAL_IN
- J2 pad T: SIGNAL_OUT -> Net-(C2-Pad1)
- Q201 pad 1: GND -> VCLEAN
- Q201 pad 2: Net-(C201-Pad1) -> Net-(C219-Pad2)
- Q201 pad 3: Net-(C202-Pad2) -> Net-(C217-Pad1)
- Q202 pad 1: GND -> Net-(Q202-Pad1)
- Q202 pad 2: Net-(C202-Pad1) -> Net-(C220-Pad2)
- Q202 pad 3: Net-(C203-Pad1) -> Net-(C220-Pad1)
- R1 pad 1: BYPASS_FUZZ -> Net-(R1-Pad1)
- R1 pad 2: GND -> Net-(R1-Pad2)
- R101 pad 1: Net-(C101-Pad2) -> VCLEAN
- R101 pad 2: FUZZ_OUT -> Net-(C102-Pad1)
- R102 pad 2: Net-(C101-Pad1) -> Net-(C103-Pad1)
- R103 pad 1: Net-(C101-Pad1) -> VCLEAN
- R103 pad 2: GND -> Net-(C104-Pad2)
- R104 pad 1: Net-(C103-Pad1) -> Net-(C104-Pad2)
- R104 pad 2: Net-(C102-Pad1) -> GND
- R105 pad 1: FUZZ_OUT -> Net-(R105-Pad1)
- R105 pad 2: Net-(C104-Pad1) -> Net-(Q102-Pad1)
- R106 pad 2: Net-(C104-Pad2) -> Net-(C105-Pad1)
- R107 pad 1: Net-(C104-Pad2) -> VCLEAN
- R107 pad 2: GND -> Net-(C105-Pad2)
- R108 pad 1: Net-(R108-Pad1) -> Net-(C105-Pad2)
- R108 pad 2: Net-(C105-Pad1) -> GND
- R109 pad 1: Net-(R108-Pad1) -> Net-(R109-Pad1)
- R109 pad 2: GND -> Net-(C106-Pad2)
- R2 pad 1: Net-(C2-Pad2) -> Net-(R1-Pad1)
- R2 pad 2: BYPASS_FUZZ -> Net-(R2-Pad2)
- R201 pad 1: VCLEAN -> Net-(C201-Pad2)
- R201 pad 2: Net-(C201-Pad1) -> GND
- R202 pad 1: VCLEAN -> Net-(C202-Pad1)
- R202 pad 2: Net-(C202-Pad2) -> Net-(C201-Pad1)
- R203 pad 1: Net-(C202-Pad1) -> VCLEAN
- R203 pad 2: Net-(R203-Pad2) -> Net-(C202-Pad1)
- R204 pad 1: VCLEAN -> Net-(R204-Pad1)
- R204 pad 2: Net-(C203-Pad1) -> Net-(C204-Pad2)
- R205 pad 1: Net-(R205-Pad1) -> Net-(C206-Pad1)
- R205 pad 2: Net-(R205-Pad2) -> Net-(C205-Pad1)
- R206 pad 1: Net-(D203-Pad2) -> Net-(C206-Pad1)
- R206 pad 2: Net-(C207-Pad1) -> Net-(C206-Pad2)
- R207 pad 1: Net-(D206-Pad2) -> Net-(C209-Pad2)
- R207 pad 2: VCLEAN -> Net-(C233-Pad2)
- R208 pad 1: Net-(R208-Pad1) -> Net-(C211-Pad2)
- R208 pad 2: Net-(R208-Pad2) -> Net-(C209-Pad1)
- R209 pad 1: Net-(R208-Pad1) -> Net-(C210-Pad2)
- R209 pad 2: Net-(R209-Pad2) -> Net-(C209-Pad1)
- R210 pad 1: Net-(R210-Pad1) -> Net-(C214-Pad1)
- R210 pad 2: Net-(R208-Pad1) -> Net-(C210-Pad1)
- R211 pad 1: SIGNAL_OUT -> Net-(C213-Pad1)
- R211 pad 2: Net-(R210-Pad1) -> Net-(R211-Pad2)
- R3 pad 1: Net-(C2-Pad1) -> Net-(R1-Pad1)
- R3 pad 2: GND -> Net-(R3-Pad2)
- R4 pad 1: Net-(C3-Pad2) -> Net-(R1-Pad1)
- R4 pad 2: GND -> Net-(R4-Pad2)
- R5 pad 1: VCLEAN -> Net-(R5-Pad1)
- R5 pad 2: Net-(C4-Pad1) -> Net-(R1-Pad1)
- R6 pad 1: Net-(C4-Pad1) -> Net-(R6-Pad1)
- R6 pad 2: GND -> Net-(R5-Pad1)
- R7 pad 1: VCLEAN -> Net-(R7-Pad1)
- R7 pad 2: Net-(Q2-Pad3) -> Net-(R6-Pad1)
- R8 pad 1: Net-(Q2-Pad1) -> Net-(C1-Pad1)
- R8 pad 2: GND -> Net-(R7-Pad1)
- R9 pad 1: Net-(C6-Pad2) -> Net-(C2-Pad1)
- R9 pad 2: GND -> Net-(C1-Pad1)
- RV1 pad 1: Net-(C3-Pad1) -> Net-(RV1-Pad1)
- RV1 pad 2: Net-(C8-Pad2) -> Net-(R1-Pad2)
- RV1 pad 3: Net-(C7-Pad1) -> GND
- RV101 pad 1: Net-(R114-Pad1) -> Net-(C102-Pad1)
- RV101 pad 2: Net-(C112-Pad1) -> Net-(C102-Pad1)
- RV101 pad 3: GND -> Net-(C101-Pad1)
- RV102 pad 1: Net-(C114-Pad2) -> Net-(R109-Pad1)
- RV102 pad 2: Net-(C114-Pad1) -> Net-(R109-Pad1)
- RV102 pad 3: Net-(RV102-Pad3) -> VCLEAN
- RV103 pad 3: Net-(RV103-Pad3) -> (no net)
- RV2 pad 1: Net-(C11-Pad1) -> Net-(RV2-Pad1)
- RV2 pad 2: Net-(C11-Pad2) -> Net-(R2-Pad2)
- RV2 pad 3: Net-(C11-Pad2) -> GND
- RV201 pad 1: Net-(R203-Pad2) -> Net-(R204-Pad1)
- RV201 pad 3: Net-(RV201-Pad3) -> Net-(C205-Pad2)
- RV202 pad 1: Net-(C203-Pad2) -> Net-(C210-Pad1)
- RV202 pad 2: Net-(D201-Pad2) -> Net-(R211-Pad2)
- RV202 pad 3: Net-(C204-Pad2) -> Net-(C210-Pad2)
- RV203 pad 1: GND -> Net-(C211-Pad1)
- RV203 pad 2: Net-(RV203-Pad2) -> Net-(R213-Pad2)
- RV203 pad 3: Net-(D203-Pad2) -> Net-(C211-Pad2)
- RV204 pad 1: Net-(RV204-Pad1) -> Net-(C214-Pad1)
- RV204 pad 2: Net-(R208-Pad2) -> Net-(C212-Pad2)
- RV204 pad 3: Net-(RV204-Pad3) -> Net-(C209-Pad1)
- RV205 pad 2: Net-(R209-Pad2) -> Net-(R249-Pad2)
- RV205 pad 3: Net-(RV205-Pad3) -> GND
- RV3 pad 1: Net-(R20-Pad1) -> Net-(RV3-Pad1)
- RV3 pad 2: Net-(R20-Pad1) -> Net-(R3-Pad2)
- RV3 pad 3: Net-(R21-Pad2) -> GND
- RV4 pad 2: Net-(C18-Pad1) -> Net-(R4-Pad2)
- SW1 pad 1: Net-(D6-Pad1) -> (no net)
- SW1 pad 2: Net-(R20-Pad1) -> Net-(RV1-Pad1)
- SW1 pad 3: Net-(D3-Pad1) -> SIGNAL_IN
- SW101 pad 2: Net-(SW101-Pad2) -> GND
- SW101 pad 3: Net-(C106-Pad1) -> Net-(R105-Pad1)
- SW2 pad 1: Net-(RV5-Pad2) -> (no net)
- SW2 pad 2: Net-(SW2-Pad2) -> Net-(RV2-Pad1)
- SW2 pad 3: Net-(C18-Pad1) -> FUZZ_OUT
- SW201 pad 1: Net-(RV204-Pad1) -> Net-(RV205-Pad1)
- SW201 pad 2: Net-(RV203-Pad2) -> Net-(C215-Pad1)
- SW201 pad 3: Net-(SW201-Pad3) -> (no net)
- SW202 pad 1: Net-(RV205-Pad1) -> Net-(RV208-Pad1)
- SW202 pad 2: REVERB_OUT -> Net-(R243-Pad1)
- SW202 pad 3: Net-(SW202-Pad3) -> (no net)
- SW3 pad 1: BYPASS_FUZZ -> (no net)
- SW3 pad 2: FUZZ_OUT -> Net-(RV3-Pad1)
- SW3 pad 3: Net-(SW2-Pad2) -> MEGAFUCKER_OUT
- U1 pad 1: Net-(C10-Pad2) -> Net-(R5-Pad1)
- U1 pad 2: Net-(C11-Pad2) -> Net-(R1-Pad1)
- U1 pad 3: Net-(C9-Pad1) -> GND
- U1 pad 5: Net-(C10-Pad1) -> GND
- U1 pad 6: Net-(C11-Pad1) -> Net-(R6-Pad1)
- U1 pad 7: VCLEAN -> Net-(R7-Pad1)
- U1 pad 8: Net-(U1-Pad8) -> VCLEAN
- U201 pad 1: Net-(R205-Pad1) -> Net-(C203-Pad1)
- U201 pad 2: Net-(D201-Pad2) -> Net-(C203-Pad2)
- U201 pad 3: Net-(C204-Pad1) -> Net-(C202-Pad1)
- U201 pad 5: Net-(C207-Pad2) -> VCLEAN
- U201 pad 6: VCLEAN -> Net-(C206-Pad1)
- U201 pad 7: Net-(C205-Pad2) -> Net-(C206-Pad2)
- U201 pad 8: Net-(R205-Pad2) -> VCLEAN
- U202 pad 1: Net-(R210-Pad1) -> Net-(C214-Pad1)
- U202 pad 2: Net-(R208-Pad1) -> Net-(C213-Pad1)
- U202 pad 3: GND -> VCLEAN
- U202 pad 5: GND -> Net-(R216-Pad2)
- U202 pad 6: Net-(R210-Pad1) -> VCLEAN
- U202 pad 7: SIGNAL_OUT -> VCLEAN
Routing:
- net BYPASS_FUZZ: track 155.9 -> 0.00 mm
- net SIGNAL_IN: track 0.00 -> 125.3 mm
- net Net-(C214-Pad1): track 0.00 -> 120.7 mm
- net Net-(C213-Pad1): track 0.00 -> 118.0 mm, vias 0 -> 2
- net Net-(C210-Pad2): track 0.00 -> 107.9 mm
- net GND: track 129.1 -> 23.1 mm, vias 20 -> 7
- net Net-(C225-Pad1): track 0.00 -> 100.0 mm, vias 0 -> 1
- net Net-(C224-Pad1): track 0.00 -> 80.7 mm
- net Net-(C2-Pad1): track 8.89 -> 89.2 mm
- net MEGAFUCKER_OUT: track 0.00 -> 76.6 mm, vias 0 -> 1
- net Net-(C201-Pad1): track 76.8 -> 2.54 mm
- net 4.5V: track 0.00 -> 68.4 mm
- net VCLEAN: track 420.4 -> 487.2 mm, vias 0 -> 1
- net FUZZ_OUT: track 118.8 -> 52.1 mm
- net SAW_OUT: track 0.00 -> 62.0 mm
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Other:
- board size 134 x 101.6 mm -> 182.9 x 99.1 mm
- net class VCLEAN: trace_width 0.4826 -> 0.508
- board text removed: "S"
- board text removed: "T"
- board text removed: "designed by sam blake, with much love and support from ben mcdaniels and corwin jones"
